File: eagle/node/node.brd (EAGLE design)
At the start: 44.4 x 65.7 mm, 19 parts, among them IC2 7805TV, X1 MKDSN1,5/2-5,08, X2 MKDSN1,5/2-5,08, X3 MKDSN1,5/2-5,08, X4 MKDSN1,5/2-5,08, X5 MKDSN1,5/3-5,08, X6 MKDSN1,5/3-5,08

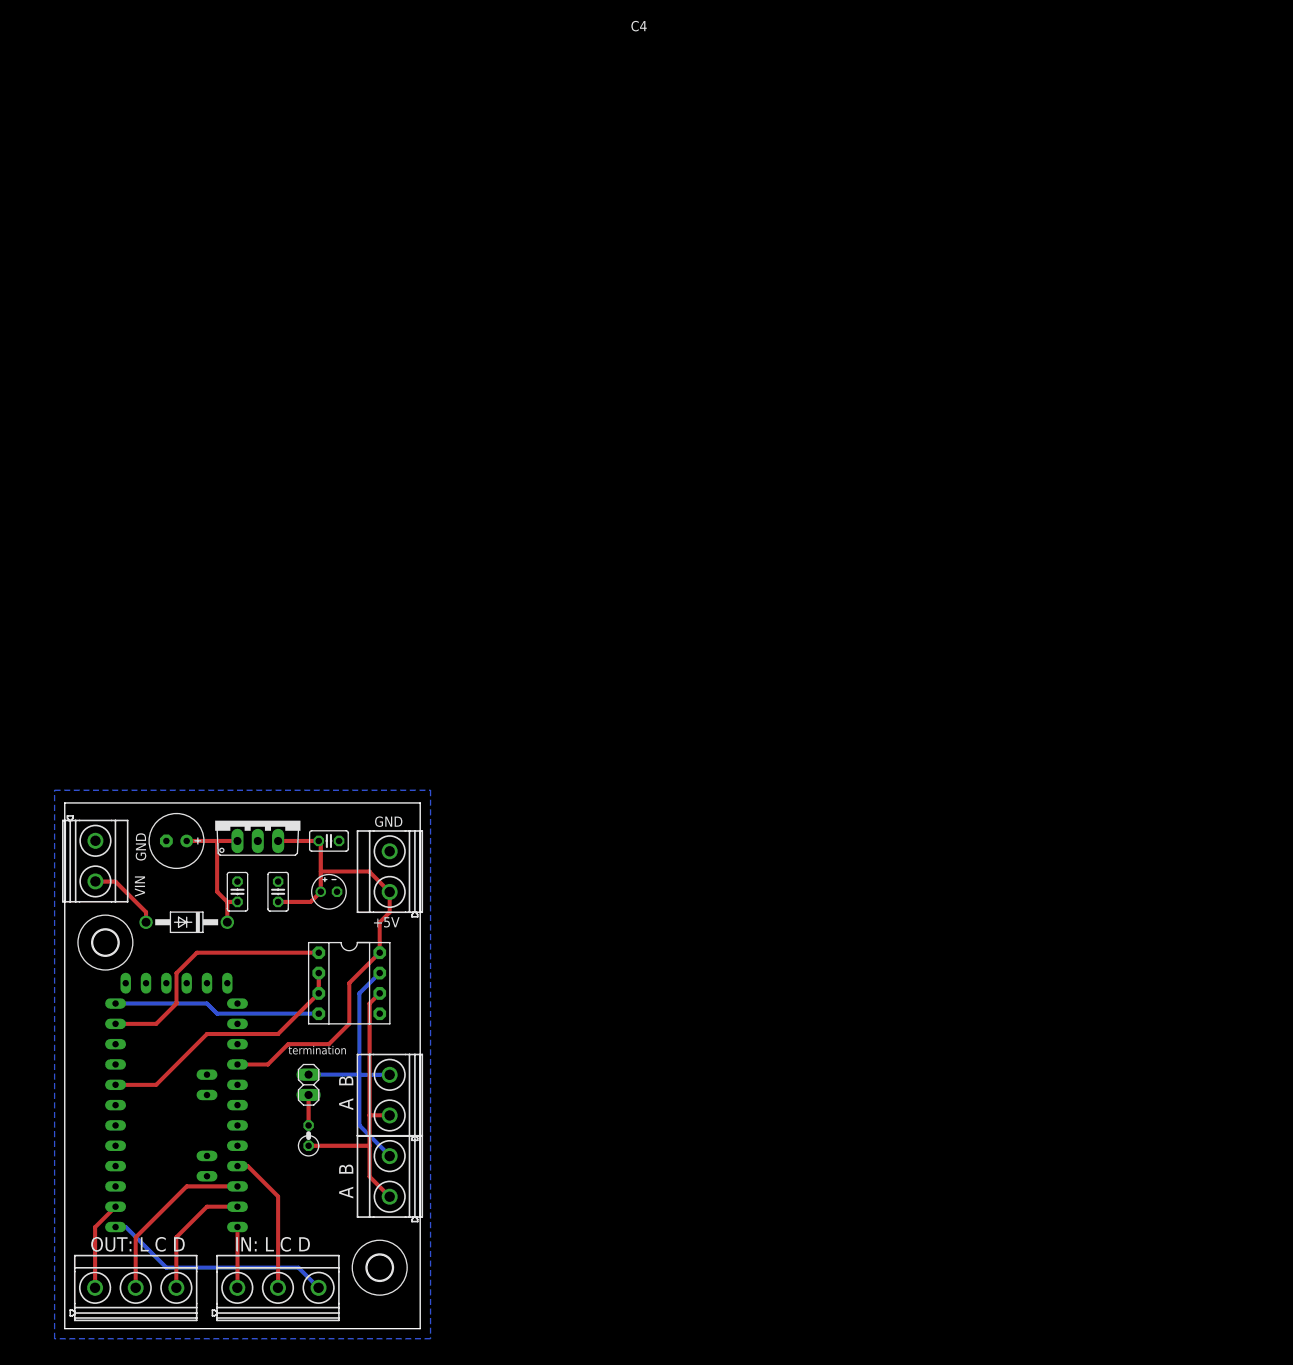
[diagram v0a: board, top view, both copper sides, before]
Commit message: periodic check in - everything working so far with breadboards.
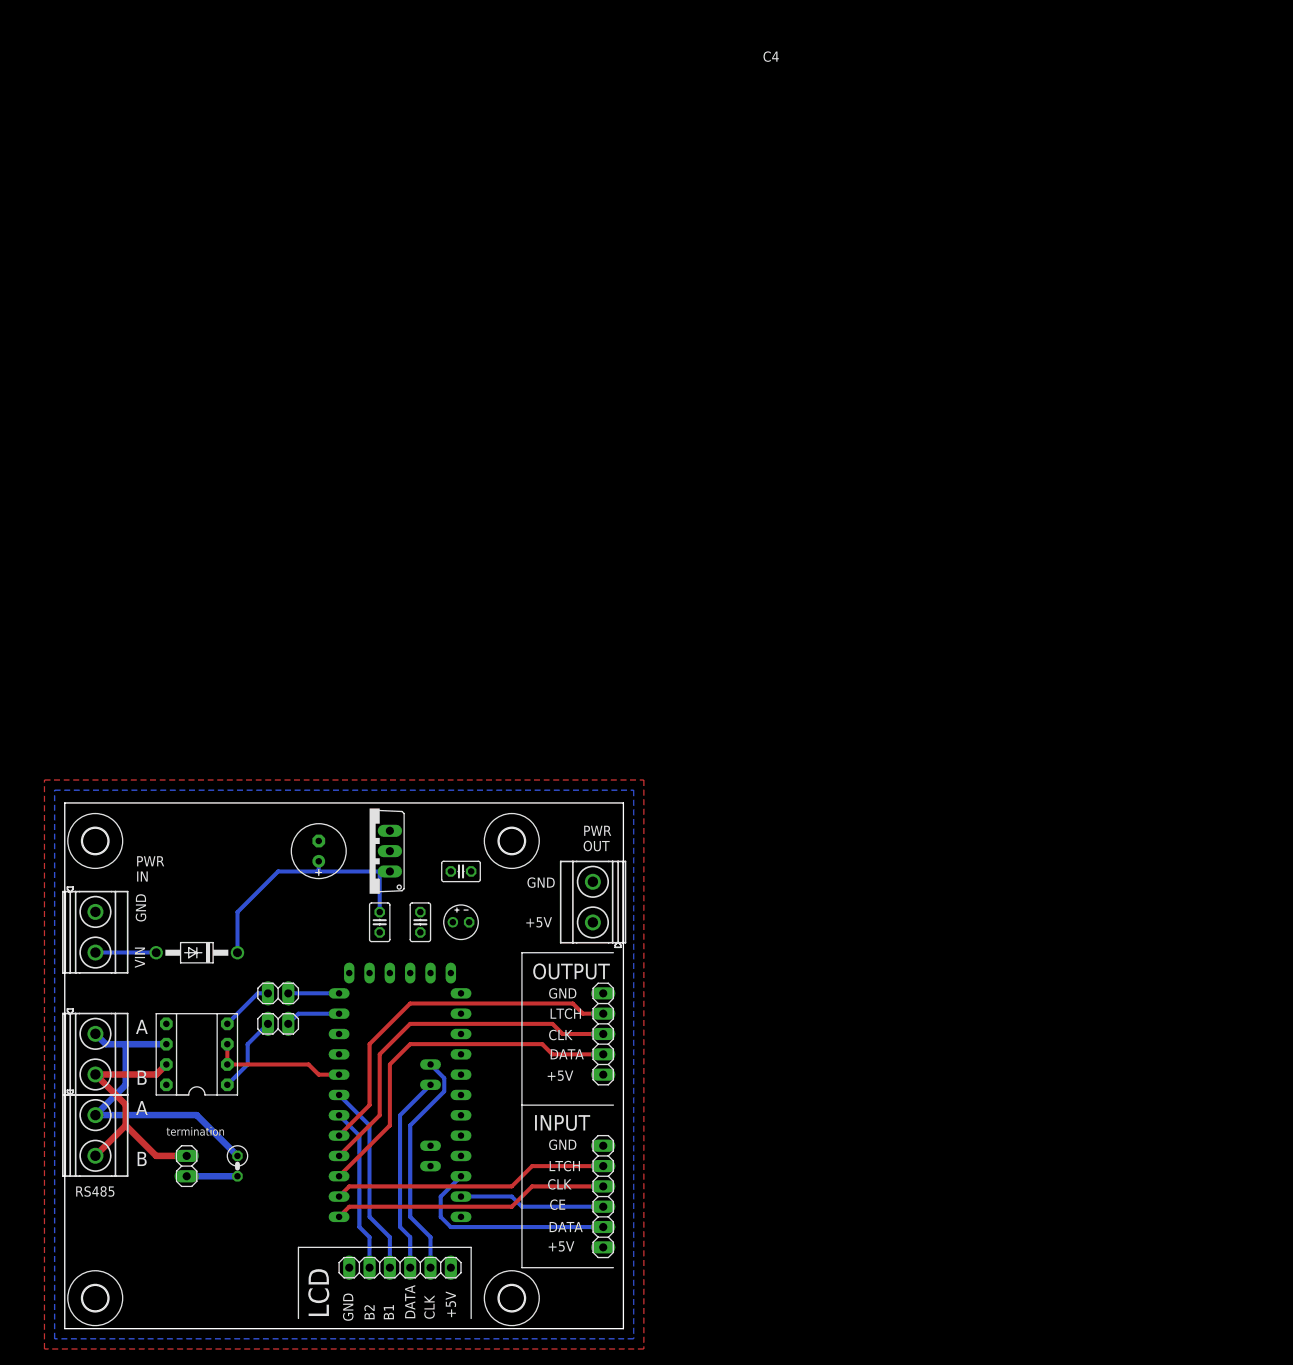
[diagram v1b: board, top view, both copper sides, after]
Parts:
- removed X5, X6: MKDSN1,5/3-5,08, con-phoenix-508:MKDSN1,5/3-5,08
- added H3, H4: MOUNT-HOLE3.2, holes:3,2
- added JP2, JP6: (no value), pinhead:1X06
- added JP3: (no value), pinhead:1X05
- added JP4, JP5: (no value), pinhead:1X02
- moved H2 52.4 mm to (55.9, 61.0)
- moved X2 37.2 mm to (3.81, 34.3), turned to 270 degrees
- moved X3 37.2 mm to (3.81, 24.1), turned to 270 degrees
- moved U$1 28.0 mm to (43.2, 29.2)
- moved X4 25.7 mm to (66.0, 53.3)
- moved U$3 21.0 mm to (16.5, 34.3), turned to 90 degrees
- moved JP1 18.3 mm to (15.2, 20.3)
- moved C9 18.2 mm to (44.5, 50.8)
- moved C8 18.2 mm to (39.4, 50.8), turned to 270 degrees
- moved C3 17.8 mm to (31.8, 59.7), turned to 90 degrees
- moved H1 16.9 mm to (55.9, 3.81)
- moved C10 16.9 mm to (49.5, 57.1)
- moved C4 16.9 mm to (49.5, 50.8)
- moved IC2 14.5 mm to (38.1, 59.7), turned to 90 degrees
- moved R1 9.67 mm to (21.6, 20.3), turned to 270 degrees
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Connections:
- new net ICE: JP2.3, U$1.D11
- new net LB1: JP6.4, U$1.D3
- new net LB2: JP6.5, U$1.D4
- new net LCLOCK: JP6.2, U$1.A5
- new net LDATA: JP6.3, U$1.A4
- new net N$10: JP5.2, U$3.4
- new net N$11: JP4.1, U$3.1
- net DI: now also JP5.1; no longer U$3.4
- net GND: now also JP2.6, JP3.5, JP6.6
- net ICLOCK: now also JP2.4, U$1.D9; no longer U$1.D13, X5.2
- net IDATA: now also JP2.2, U$1.D12; no longer U$1.D9, X5.3
- net ILATCH: now also JP2.5, U$1.D8; no longer U$1.D10, X5.1
- net OCLOCK: now also JP3.3, U$1.D6; no longer U$1.D12, X6.2
- net ODATA: now also JP3.2, U$1.D7; no longer U$1.D11, X6.3
- net OLATCH: now also JP3.4, U$1.D5; no longer U$1.D8, X6.1
- net RO: now also JP4.2; no longer U$3.1
- net VCC: now also JP2.1, JP3.1, JP6.1
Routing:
- net VCC: track 61.8 -> 0.00 mm
- net OLATCH: track 11.2 -> 44.8 mm
- net ODATA: track 15.5 -> 44.8 mm
- net LCLOCK: track 0.00 -> 28.9 mm
- net ILATCH: track 7.60 -> 34.6 mm
- net LDATA: track 0.00 -> 25.0 mm
- net RO: track 31.3 -> 6.88 mm
- net LB1: track 0.00 -> 24.2 mm
- net OCLOCK: track 21.7 -> 44.8 mm
- net LB2: track 0.00 -> 20.6 mm
- net DI: track 25.9 -> 6.35 mm
- net ICE: track 0.00 -> 18.3 mm
- net ICLOCK: track 18.1 -> 34.6 mm
- net DE: track 32.7 -> 17.0 mm
- net N$1: track 18.3 -> 33.9 mm
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- added copper zone on layer 1, net VCC
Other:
- board size 44.4 x 65.7 mm -> 69.8 x 65.7 mm
- board text added: "A"
- board text added: "B"
- board text added: "B1"
- board text added: "B2"
- board text added: "CE"
- board text added: "CLK"
- board text added: "DATA"
- board text added: "INPUT"
- board text added: "LCD"
- board text added: "LTCH"
- board text added: "Node 8/19"
- board text added: "OUTPUT"
- board text added: "PWR IN"
- board text added: "PWR OUT"
- board text added: "RS485"
- board text removed: "A B"
- board text removed: "IN: L C D"
- board text removed: "Node 7/19"
- board text removed: "OUT: L C D"

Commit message: periodic check-in
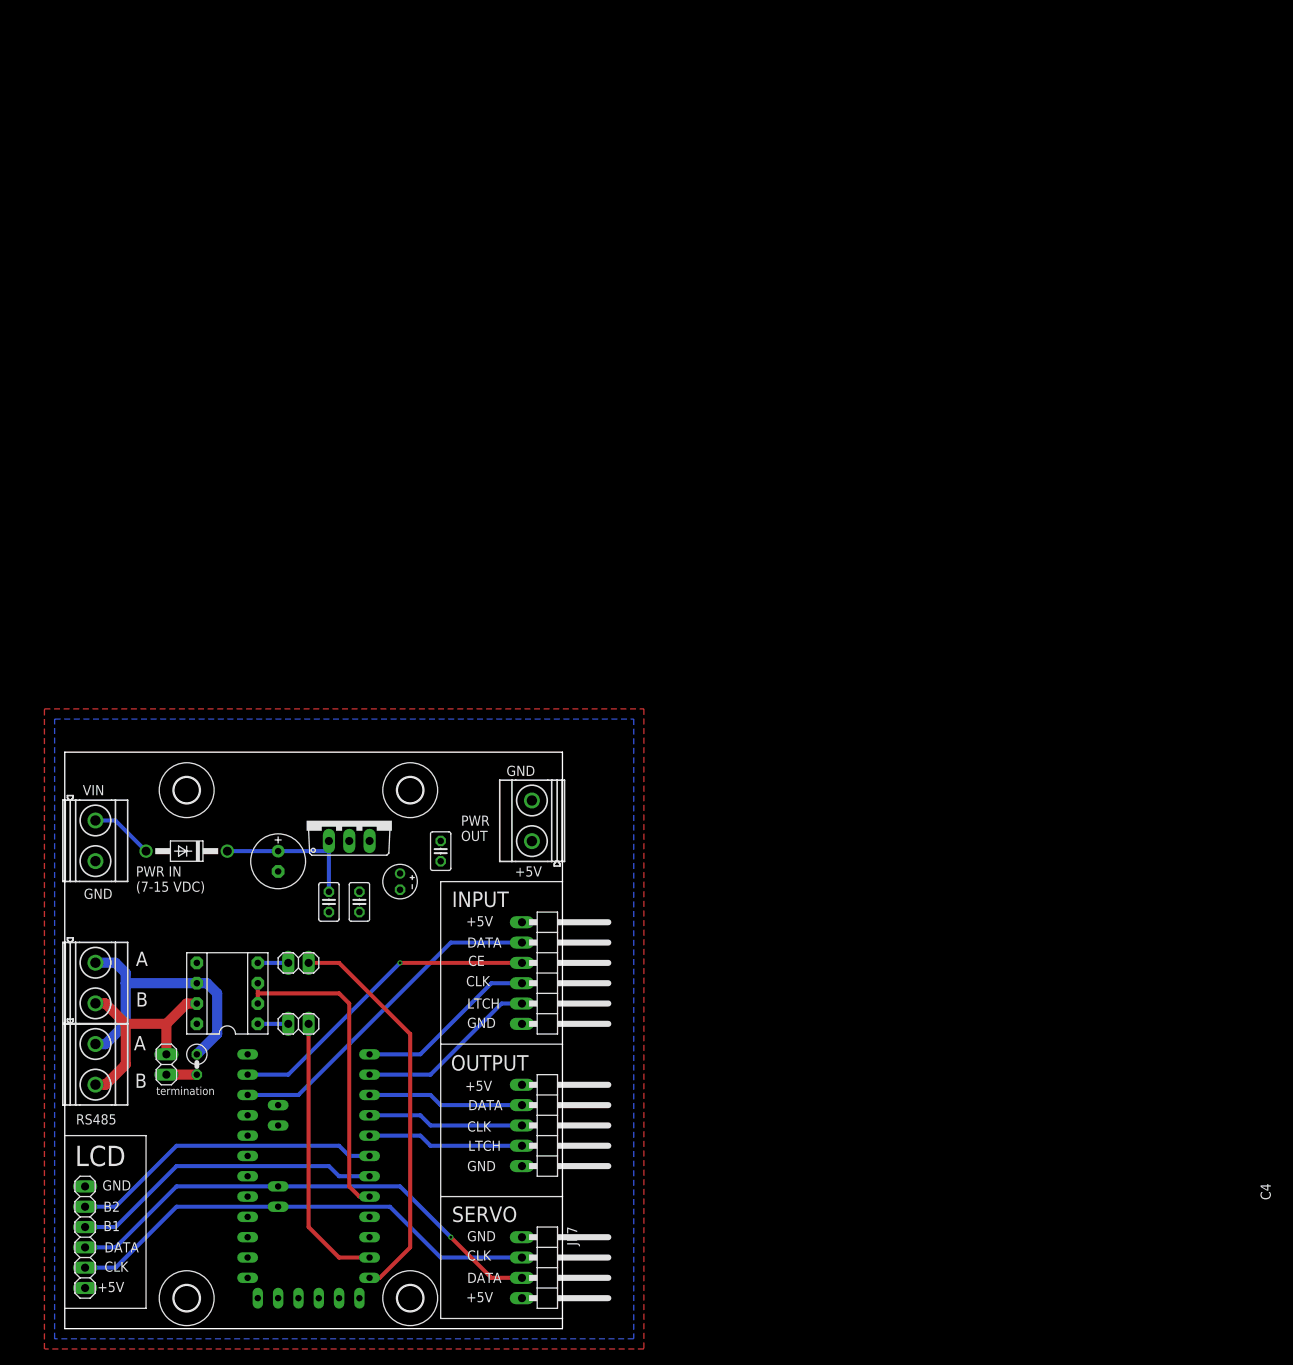
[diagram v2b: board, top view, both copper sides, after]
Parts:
- added JP7: (no value), pinhead:1X04/90
- JP2: device pinhead:1X06 -> pinhead:1X06/90
- JP3: device pinhead:1X05 -> pinhead:1X05/90
- moved H1 40.6 mm to (15.2, 3.81)
- moved JP6 39.6 mm to (2.54, 11.4), turned to 90 degrees
- moved H3 39.4 mm to (43.2, 3.81)
- moved JP2 28.7 mm to (61.0, 44.5), turned to 270 degrees
- moved U$1 17.3 mm to (29.2, 19.1), turned to 180 degrees
- moved H2 14.2 mm to (43.2, 67.3)
- moved R1 13.7 mm to (16.5, 33.0)
- moved H4 13.1 mm to (15.2, 67.3)
- moved JP3 13.1 mm to (61.0, 25.4), turned to 270 degrees
- moved JP1 13.0 mm to (12.7, 33.0)
- moved D1 12.8 mm to (15.2, 59.7)
- moved X4 12.7 mm to (58.4, 63.5)
- moved X1 11.4 mm to (3.81, 61.0)
- moved C4 9.16 mm to (41.9, 55.9), turned to 270 degrees
- moved X3 8.89 mm to (3.81, 33.0)
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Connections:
- removed net LCLOCK: JP6.2, U$1.A5
- removed net LDATA: JP6.3, U$1.A4
- new net SCL: JP6.2, JP7.2, U$1.A5
- new net SDA: JP6.3, JP7.3, U$1.A4
- net GND: now also JP7.1, X1.2; no longer X1.1
- net N$2: now also X1.1; no longer X1.2
- net VCC: now also JP7.4
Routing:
- net SDA: track 0.00 -> 62.5 mm, vias 0 -> 1
- net SCL: track 0.00 -> 60.4 mm
- net DI: track 6.35 -> 49.7 mm
- net LCLOCK: track 28.9 -> 0.00 mm
- net RO: track 6.88 -> 34.6 mm
- net OLATCH: track 44.8 -> 19.6 mm
- net OCLOCK: track 44.8 -> 19.6 mm
- net ODATA: track 44.8 -> 19.6 mm
- net LDATA: track 25.0 -> 0.00 mm
- net DE: track 17.0 -> 40.4 mm
- net ICE: track 18.3 -> 40.1 mm, vias 0 -> 1
- net LB2: track 20.6 -> 39.2 mm
- net IDATA: track 27.0 -> 42.2 mm
- net LB1: track 24.2 -> 39.2 mm
- net N$1: track 33.9 -> 19.1 mm
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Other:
- board size 69.8 x 65.7 mm -> 62.2 x 72.1 mm
- board text added: "Node 9/19"
- board text added: "PWR IN (7-15 VDC)"
- board text added: "SERVO"
- board text removed: "Node 8/19"
- board text removed: "PWR IN"
